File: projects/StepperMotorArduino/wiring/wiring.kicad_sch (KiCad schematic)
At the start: 6 parts, among them M1 Stepper_Motor_bipolar, SW1 Limit switch (left), SW2 Limit switch (right)

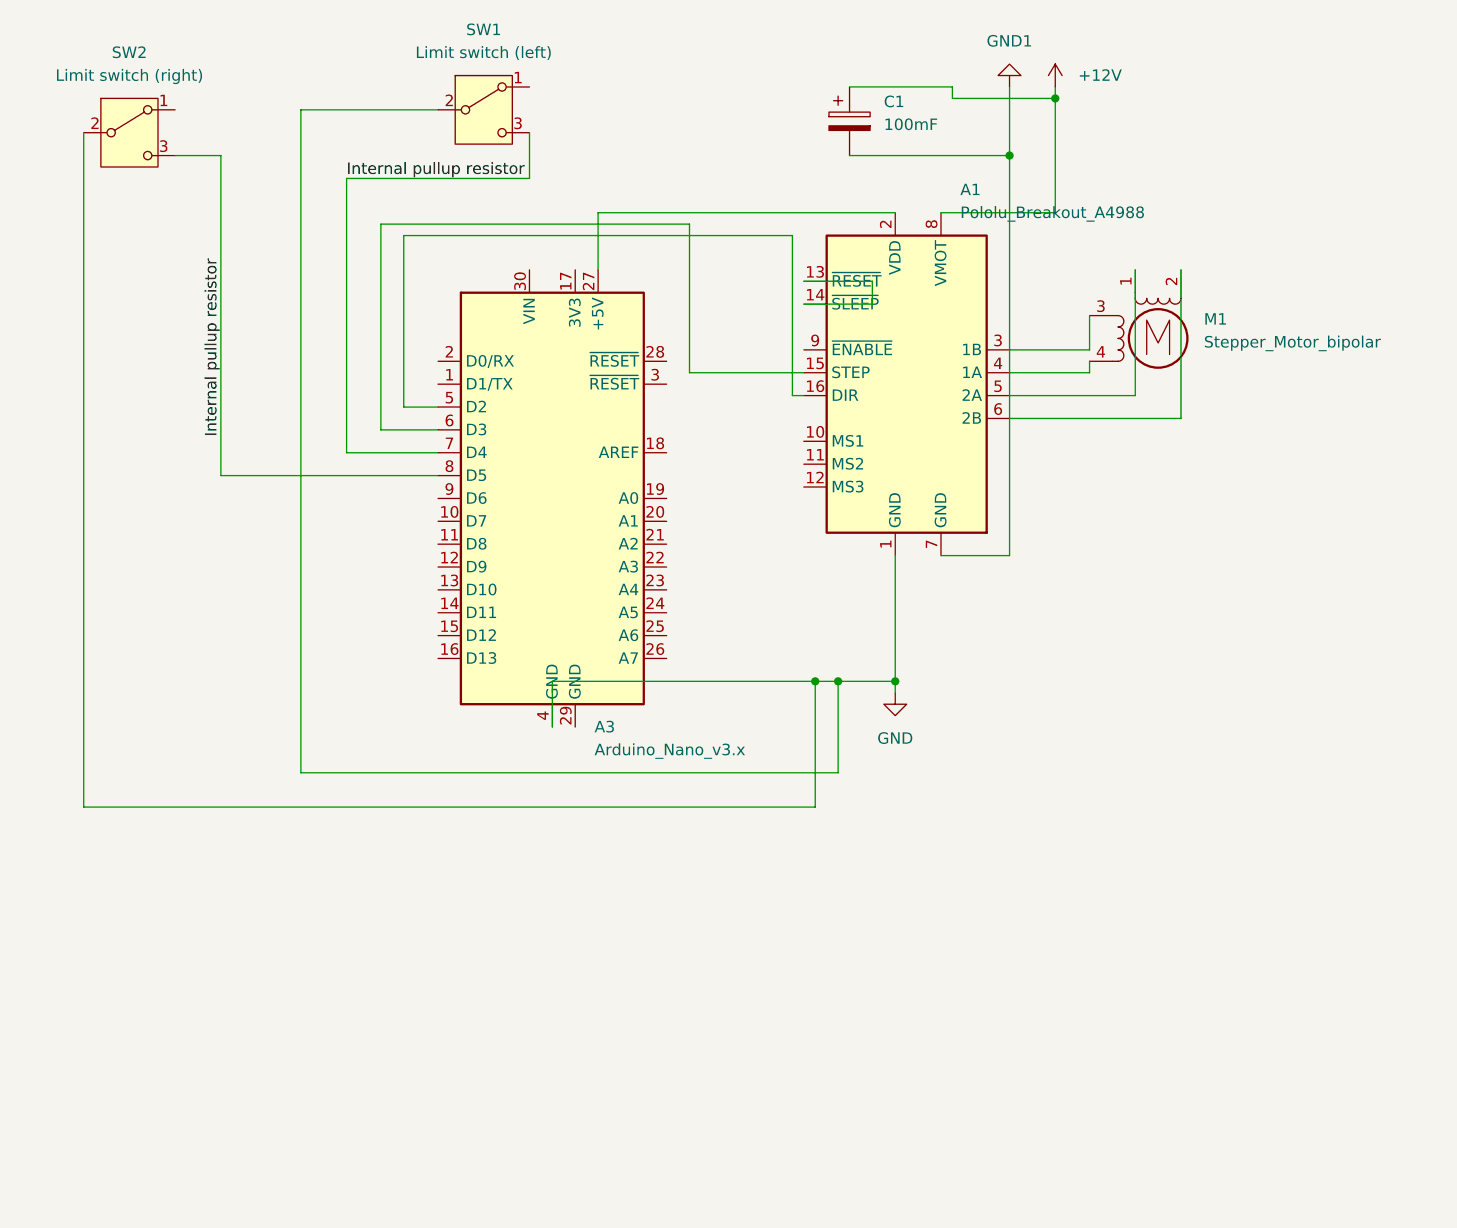
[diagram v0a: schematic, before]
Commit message: Progress
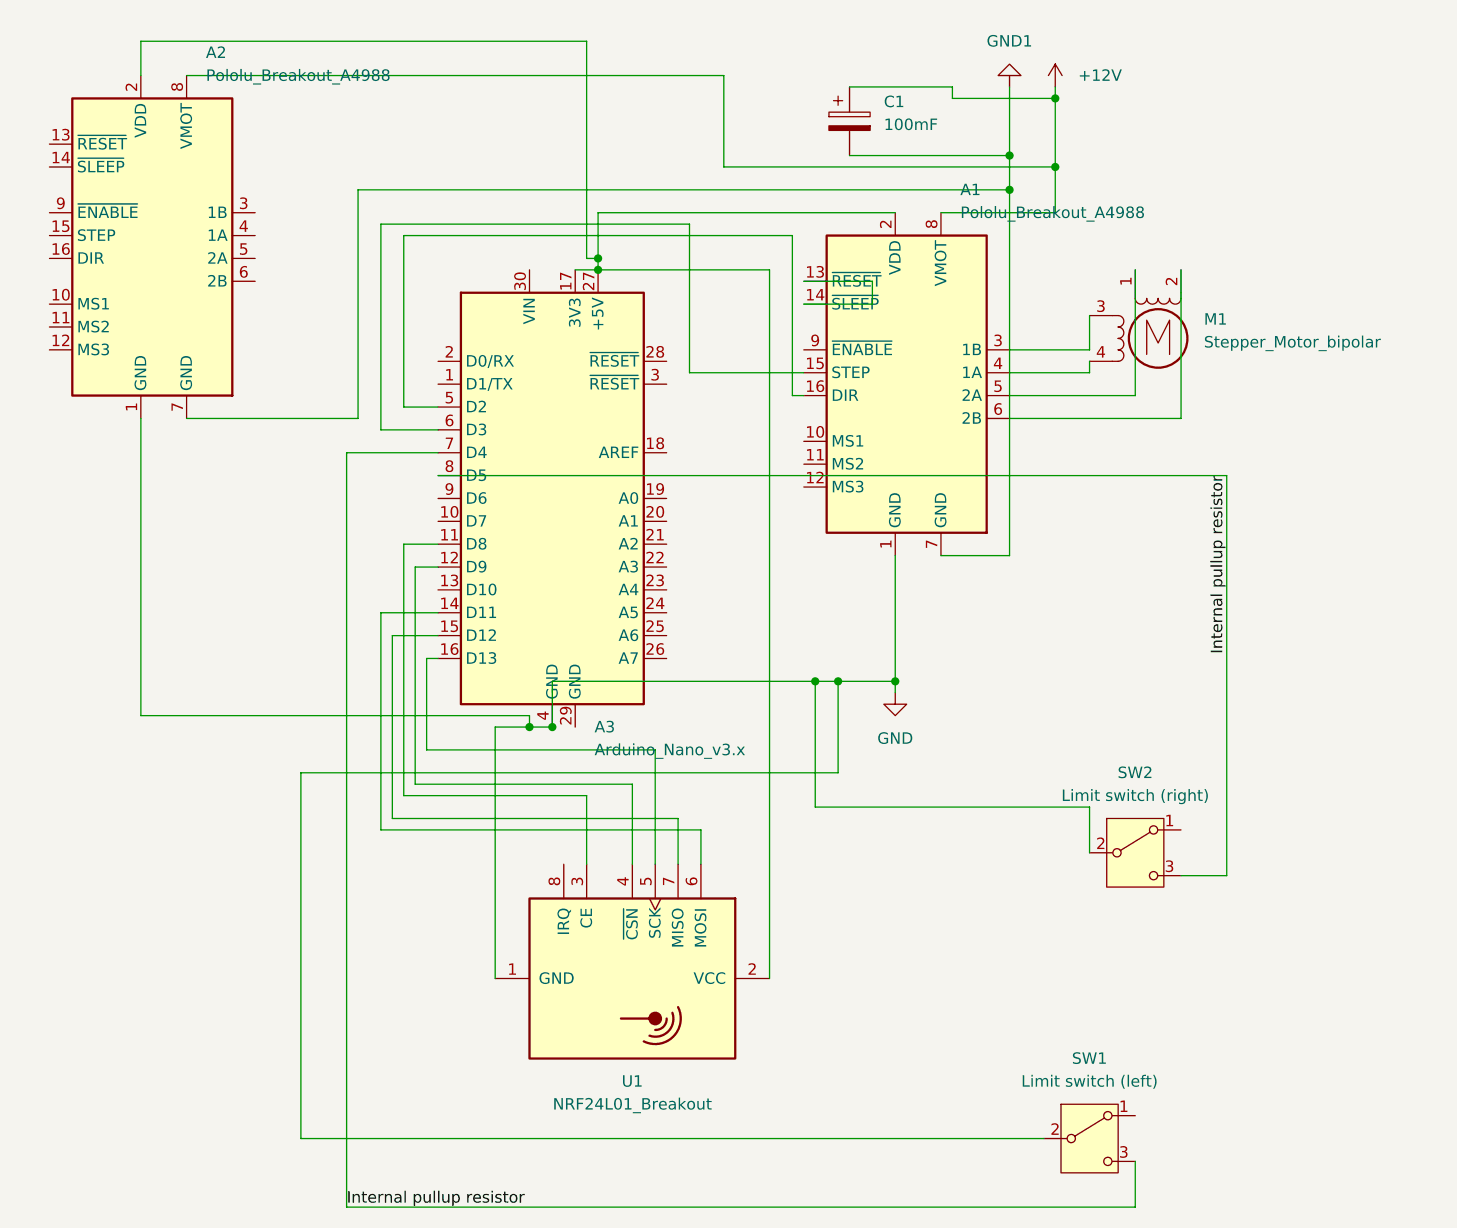
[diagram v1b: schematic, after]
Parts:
- added A2: Pololu_Breakout_A4988, Module:Pololu_Breakout-16_15.2x20.3mm, symbol Driver_Motor:Pololu_Breakout_A4988
- added U1: NRF24L01_Breakout, RF_Module:nRF24L01_Breakout, symbol RF:NRF24L01_Breakout
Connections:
- net +12V: now also A2.8 (VMOT)
- net GND: now also A2.1 (GND), U1.1 (GND)
- net GND1: now also A2.7 (GND)
- net at A3.11 (D8): now also U1.3 (CE)
- net at A3.12 (D9): now also U1.4 (~{CSN})
- net at A3.14 (D11): now also U1.6 (MOSI)
- net at A3.15 (D12): now also U1.7 (MISO)
- net at A3.16 (D13): now also U1.5 (SCK)
- net at A3.17 (3V3): now also A1.2 (VDD), A3.27 (+5V), A2.2 (VDD), U1.2 (VCC)
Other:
- moved on the sheet: SW1, SW2
